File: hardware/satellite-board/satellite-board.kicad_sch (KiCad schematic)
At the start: 27 parts, among them J1 MTJ-88ARX1-FSM-LG, J2 B2B-PH-K-S, Q1 MMBT3904, U1 LORA1262-915TCXO, U2 XC6220B331MR, U3 ESP32-C6-DEVKITC-1-N8, U4 MAX3485

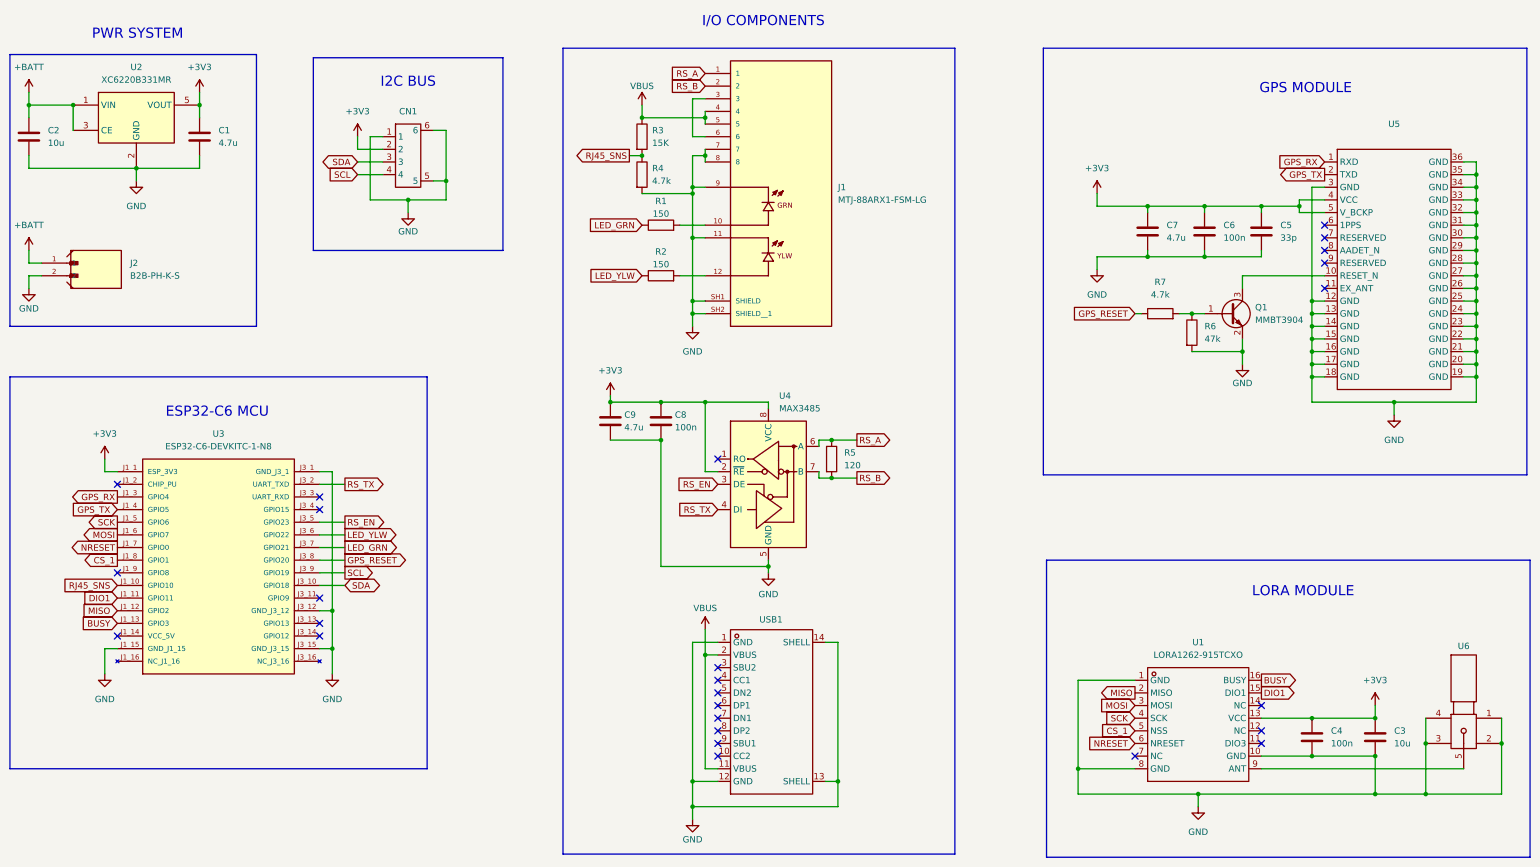
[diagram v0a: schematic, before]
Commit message: Branch updates
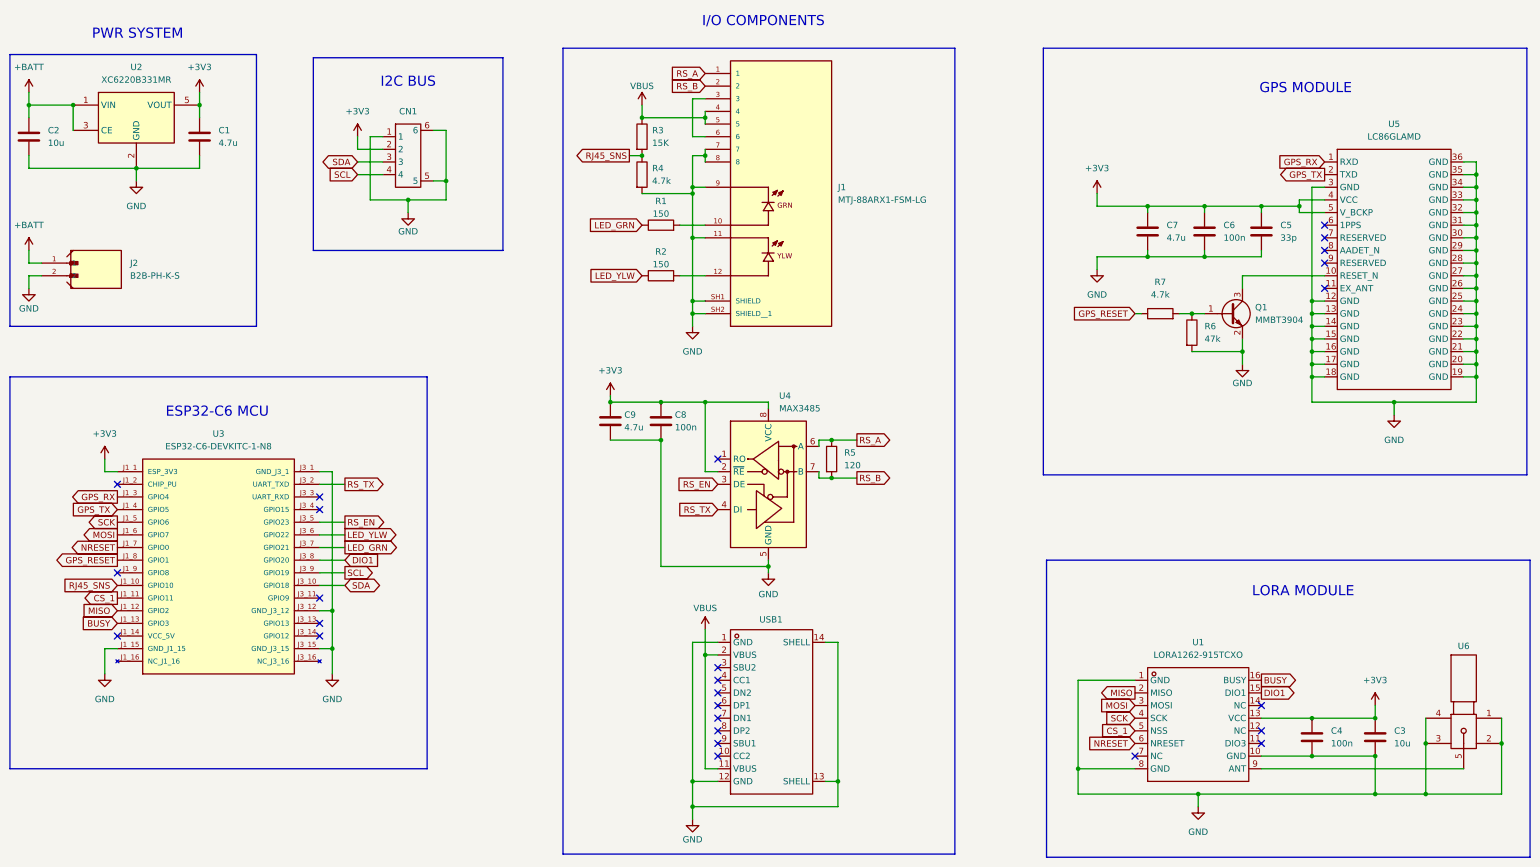
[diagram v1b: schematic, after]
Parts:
- CN1: value ~ -> XY-SM04B-SRSS-TB; LCSC (none) -> C51940130
- U5: value ~ -> LC86GLAMD
- U6: value ~ -> SMA-KWE
- USB1: value ~ -> TYPE-C 16PIN 2MD(073)
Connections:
- net CS_1: now also U3.J1_11 (GPIO11); no longer U3.J1_8 (GPIO1)
- net DIO1: now also U3.J3_8 (GPIO20); no longer U3.J1_11 (GPIO11)
- net GPS_RESET: now also U3.J1_8 (GPIO1); no longer U3.J3_8 (GPIO20)
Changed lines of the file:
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@@
 	(wire
 		(pts
+			(xy 123.19 161.29) (xy 118.11 161.29)
+		)
+		(stroke
+			(width 0)
+			(type default)
+		)
+	)
+	(wire
+		(pts
 			(xy 193.04 177.8) (xy 193.04 205.74)
 		)
@@
 	(wire
 		(pts
-			(xy 118.11 161.29) (xy 123.19 161.29)
-		)
-		(stroke
-			(width 0)
-			(type default)
-		)
-	)
-	(wire
-		(pts
 			(xy 274.32 87.63) (xy 274.32 90.17)
 		)
@@
 	(global_label "DIO1"
 		(shape input)
-		(at 77.47 168.91 180)
+		(at 123.19 161.29 0)
 		(fields_autoplaced yes)
 		(effects
@@
 				(size 1.27 1.27)
 			)
-			(justify right)
+			(justify left)
 		)
 		(property "Intersheetrefs" "${INTERSHEET_REFS}"
-			(at 70.07 168.91 0)
+			(at 130.59 161.29 0)
 			(effects
 				(font
 					(size 1.27 1.27)
 				)
-				(justify right)
+				(justify left)
 				(hide yes)
 			)
@@
 	(global_label "CS_1"
 		(shape output)
-		(at 77.47 161.29 180)
+		(at 77.47 168.91 180)
 		(fields_autoplaced yes)
 		(effects
@@
 		)
 		(property "Intersheetrefs" "${INTERSHEET_REFS}"
-			(at 69.8282 161.29 0)
+			(at 69.8282 168.91 0)
 			(effects
 				(font
@@
 	(global_label "GPS_RESET"
 		(shape output)
-		(at 123.19 161.29 0)
+		(at 77.47 161.29 180)
 		(fields_autoplaced yes)
 		(effects
@@
 				(size 1.27 1.27)
 			)
-			(justify left)
+			(justify right)
 		)
 		(property "Intersheetrefs" "${INTERSHEET_REFS}"
-			(at 136.6374 161.29 0)
+			(at 64.0226 161.29 0)
 			(effects
 				(font
 					(size 1.27 1.27)
 				)
-				(justify left)
+				(justify right)
 				(hide yes)
 			)
@@
 			)
 		)
-		(property "Value" "~"
+		(property "Value" "TYPE-C 16PIN 2MD(073)"
 			(at 208.915 172.72 0)
 			(effects
@@
 			)
 		)
-		(property "Value" "~"
+		(property "Value" "SMA-KWE"
 			(at 347.98 177.8 90)
 			(effects
@@
 			)
 		)
-		(property "Value" "~"
+		(property "Value" "LC86GLAMD"
 			(at 334.01 76.2 0)
 			(effects
@@
 			)
 		)
-		(property "Value" "~"
+		(property "Value" "XY-SM04B-SRSS-TB"
 			(at 135.89 71.12 0)
 			(effects
@@
 			)
 		)
-		(property "LCSC" "~"
+		(property "LCSC" "C51940130"
 			(at 135.89 80.01 0)
 			(effects
